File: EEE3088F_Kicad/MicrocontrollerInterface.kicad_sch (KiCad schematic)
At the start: 44 parts, among them J1 USB_B_Micro, J10 Conn_01x01, J11 Conn_01x01, J12 Conn_01x01, J13 Conn_01x01, J2 Conn_01x01, J3 Conn_01x01, J4 Conn_01x01, J5 Conn_01x01, J6 Conn_01x01, J7 Conn_01x01, J8 Conn_01x01, J9 Conn_01x01, U1 CAT24C256, U2 INTERFACE-CP2102-GMR(QFN28), U3 STM32F051C6Tx

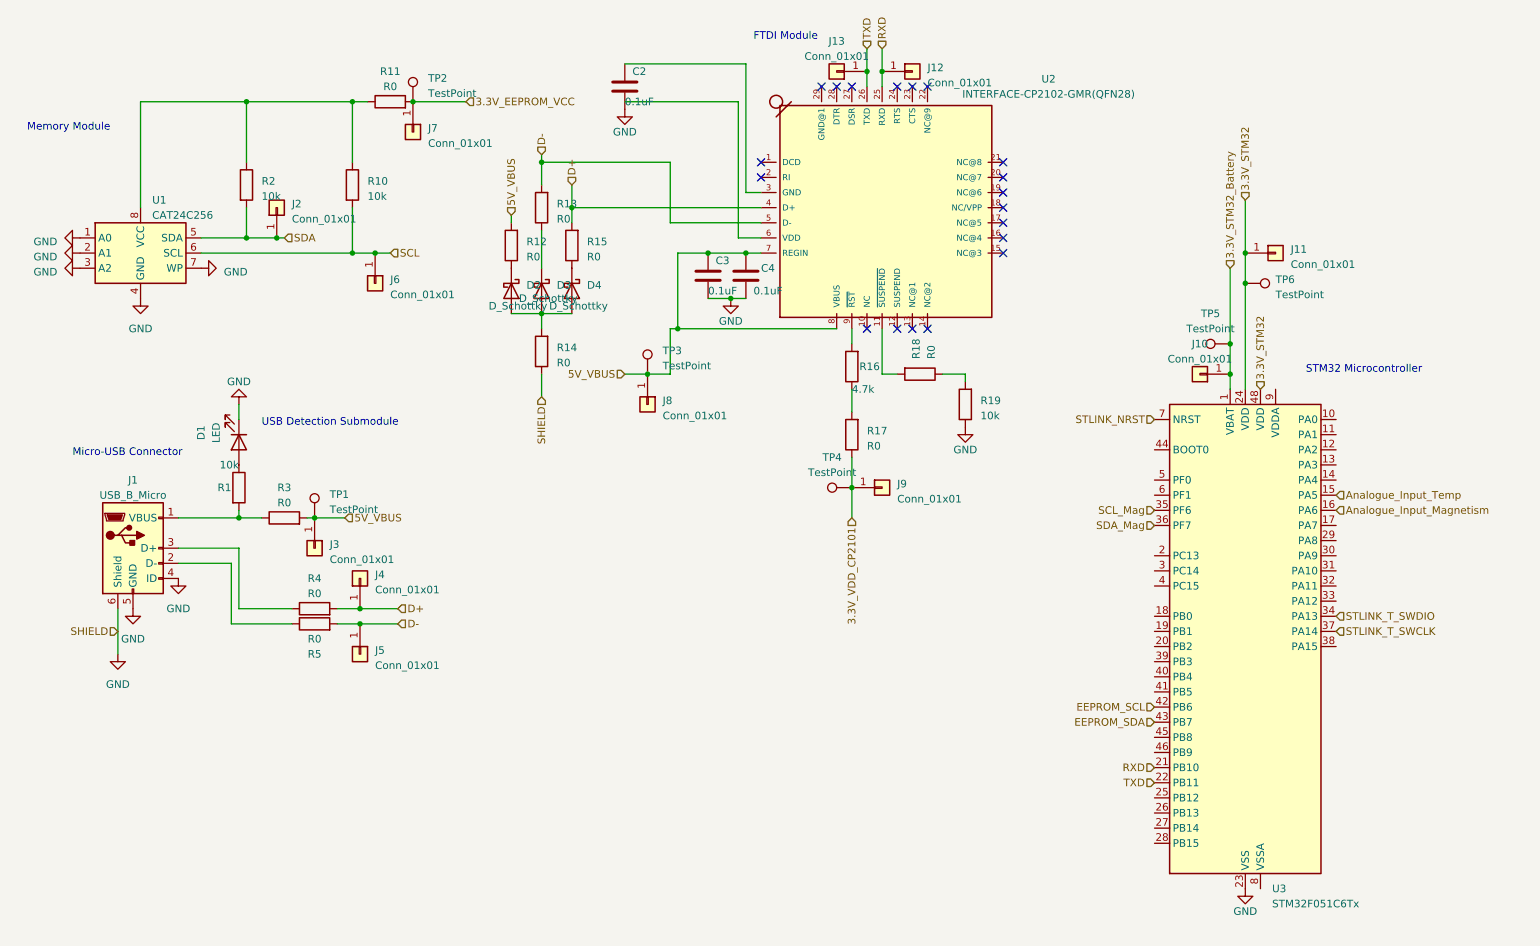
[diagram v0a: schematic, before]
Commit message: Microntroller Update
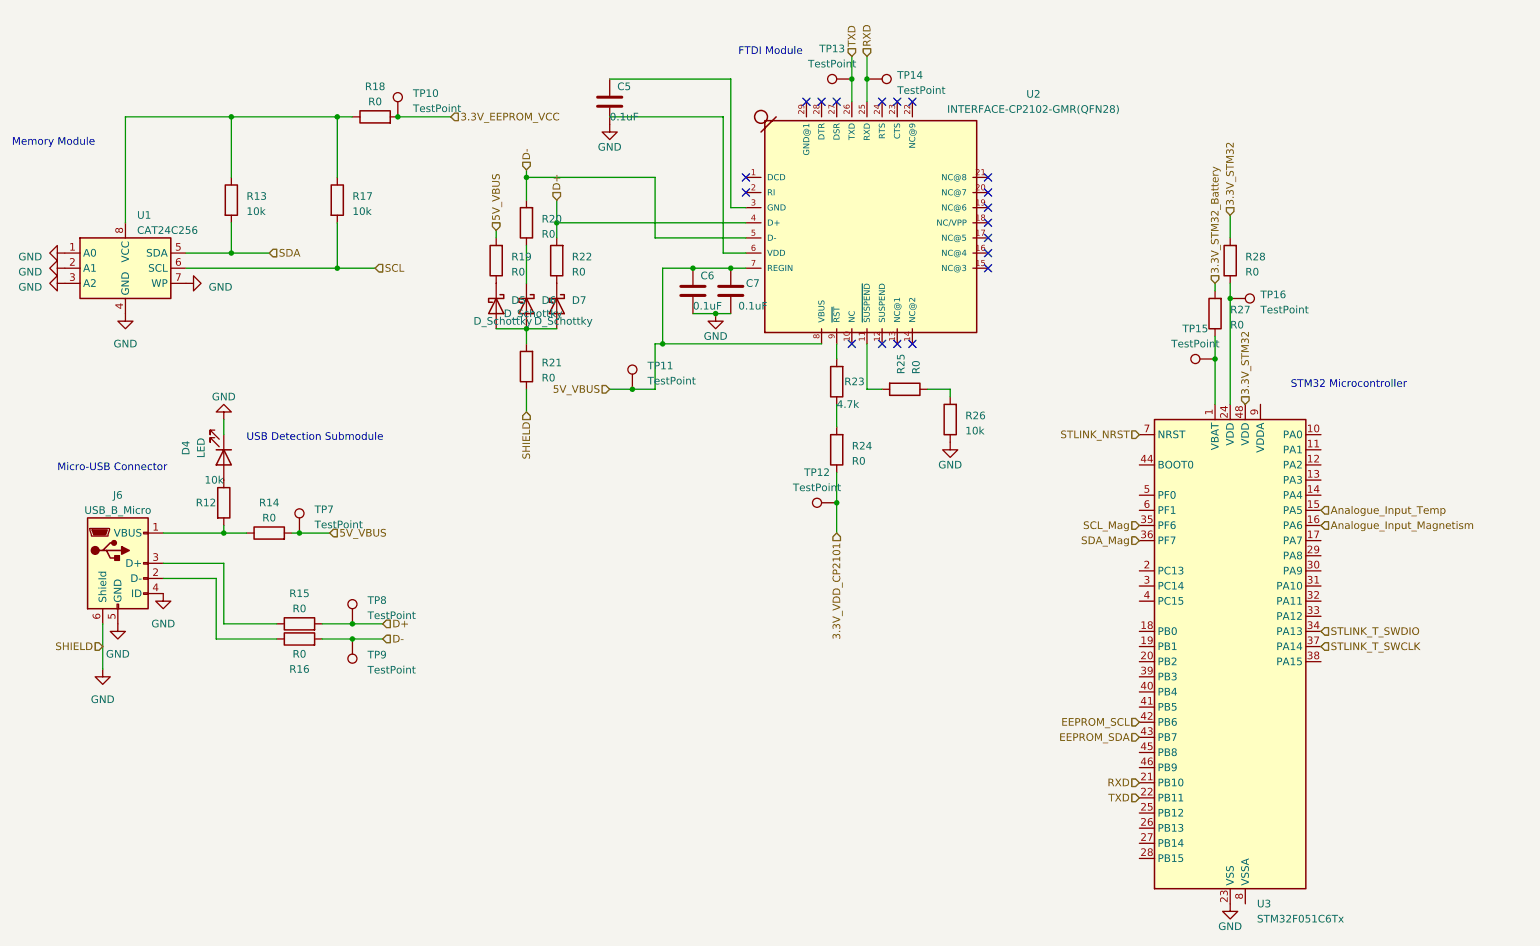
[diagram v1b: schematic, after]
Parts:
- removed C2, C3, C4: 0.1uF, symbol Device:C
- removed D1: LED, symbol Device:LED
- removed D2, D3, D4: D_Schottky, symbol Device:D_Schottky
- removed J1: USB_B_Micro, symbol Connector:USB_B_Micro
- removed J10, J11, J12, J13, J2, J3, J4, J5, J6, J7, J8, J9: Conn_01x01, symbol Connector_Generic:Conn_01x01
- removed R1, R10, R2: 10k, symbol Device:R
- removed R11, R3, R4, R5: R0, symbol Device:R
- removed TP1, TP2, TP3, TP4, TP5, TP6: TestPoint, symbol Connector:TestPoint
- added C5, C6, C7: 0.1uF, symbol Device:C
- added D4: LED, symbol Device:LED
- added D5, D6, D7: D_Schottky, symbol Device:D_Schottky
- added J6: USB_B_Micro, MICROXNJ:SHOUHAN_MICROXNJ, symbol Connector:USB_B_Micro
- added R20, R21, R22, R24, R25, R27, R28: R0, symbol Device:R
- added R23: 4.7k, symbol Device:R
- added R26: 10k, symbol Device:R
- added TP10, TP11, TP12, TP13, TP14, TP15, TP16, TP7, TP8, TP9: TestPoint, symbol Connector:TestPoint
- R12, R13, R17: value R0 -> 10k; LCSC (none) -> C17902
- R14, R15, R18: LCSC (none) -> C17888
- R16: value 4.7k -> R0; LCSC (none) -> C17888
- R19: value 10k -> R0; LCSC (none) -> C17888
- U1: footprint (none) -> EEPROM:SOIC127P600X175-8N; LCSC (none) -> C6482
- U2: footprint QFN28G_0.5-5X5MM -> USB UART Chip:QFN28G_0.5-5X5MM; LCSC (none) -> C6568
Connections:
- net 3.3V_EEPROM_VCC: now also R18.2, TP10.1
- net 3.3V_STM32: now also R28.2; no longer U3.24 (VDD)
- net 3.3V_STM32_Battery: now also R27.2; no longer U3.1 (VBAT)
- net 3.3V_VDD_CP2101: now also R24.1, TP12.1; no longer R17.1
- net 5V_VBUS: now also R14.2, R19.2, C6.1, C7.1, TP11.1, TP7.1; no longer R12.2
- net D+: now also R22.2, TP8.1
- net D-: now also R16.2, R20.2, TP9.1; no longer R13.2
- net GND: now also C5.2, C6.2, C7.2, D4.1 (K), J6.4 (ID), J6.5 (GND), J6.6 (Shield), R21.1, R26.1; no longer R14.1, R19.1
- net RXD: now also TP14.1
- net SCL: now also R17.2
- net SDA: now also R13.2
- net TXD: now also TP13.1
- net at R13.1: now also R17.1, R18.1, U1.8 (VCC)
- net at R16.1: now also J6.2 (D-); no longer R17.2
- net at U2.9 (~{RST}): now also R23.2; no longer R16.2
- net at R15.1: now also J6.3 (D+)
- net at U2.3 (GND): now also C5.1
- net at R12.1: now also D4.2 (A)
- net at U2.11 (~{SUSPEND}): now also R25.2; no longer R18.2
- new net: R27.1, TP15.1, U3.1 (VBAT)
- new net: D5.2 (A), D6.2 (A), D7.2 (A), R21.2
- new net: D5.1 (K), R19.1
- new net: R25.1, R26.2
- new net: J6.1 (VBUS), R12.2, R14.1
- new net: D7.1 (K), R22.1
- new net: R28.1, TP16.1, U3.24 (VDD)
- new net: D6.1 (K), R20.1
- new net: R23.1, R24.2
